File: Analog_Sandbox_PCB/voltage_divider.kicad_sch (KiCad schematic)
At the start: 14 parts, among them J4 PAD, J5 PAD, J6 PAD, J7 PAD

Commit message: Config LM134
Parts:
- S4: footprint Analog_Sandbox_PCB:DS-01 -> Button_Switch_THT:SW_DIP_SPSTx01_Slide_9.78x4.72mm_W7.62mm_P2.54mm

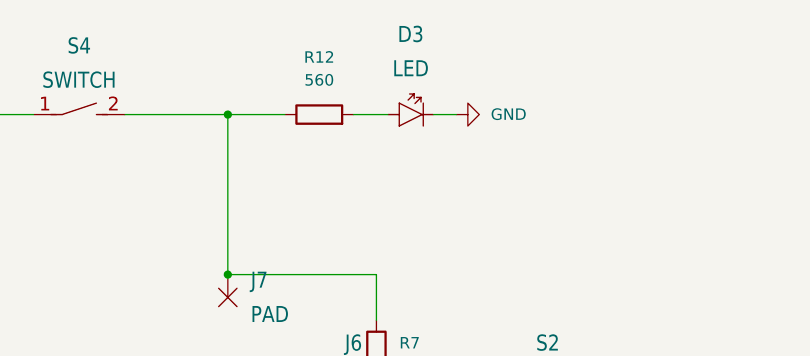
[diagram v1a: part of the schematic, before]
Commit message: All Circuits Added, Layout Almost done
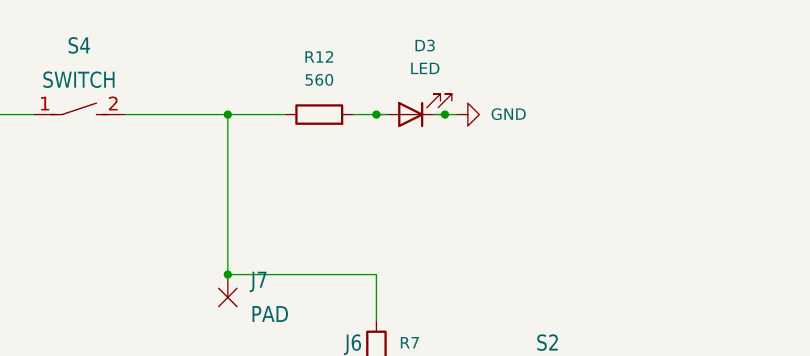
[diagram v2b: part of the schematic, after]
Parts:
- removed D3: LED, Diode_SMD:D_2010_5025Metric_Pad1.52x2.65mm_HandSolder, symbol Analog_Sandbox_PCB-eagle-import:CHIP-FLAT-Y_0603-0.35MM
- added D3: LED, Diode_SMD:D_1206_3216Metric, symbol Device:LED
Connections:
- net GND: now also D3.1 (K)
- net at R12.2: now also D3.2 (A)
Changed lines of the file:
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@@
+	)
+	(junction
+		(at 96.52 26.67)
+		(diameter 0)
+		(color 0 0 0 0)
 	)
 	(junction
@@
 	)
 	(junction
+		(at 104.14 26.67)
+		(diameter 0)
+		(color 0 0 0 0)
+	)
+	(junction
 		(at 80.01 26.67)
 		(diameter 0)
@@
 	(wire
 		(pts
-			(xy 105.41 26.67) (xy 102.87 26.67)
+			(xy 105.41 26.67) (xy 104.14 26.67)
 		)
 		(stroke
@@
 	(wire
 		(pts
+			(xy 96.52 26.67) (xy 97.79 26.67)
+		)
+		(stroke
+			(width 0)
+			(type default)
+		)
+	)
+	(wire
+		(pts
 			(xy 82.55 93.98) (xy 96.52 93.98)
 		)
@@
 	(wire
 		(pts
-			(xy 93.98 26.67) (xy 97.79 26.67)
+			(xy 93.98 26.67) (xy 96.52 26.67)
 		)
 		(stroke
@@
 		(pts
 			(xy 96.52 49.53) (xy 96.52 44.45)
+		)
+		(stroke
+			(width 0)
+			(type default)
+		)
+	)
+	(wire
+		(pts
+			(xy 104.14 26.67) (xy 102.87 26.67)
 		)
 		(stroke
@@
 			)
 			(justify right)
-		)
-	)
-	(symbol
-		(lib_id "Analog_Sandbox_PCB-eagle-import:CHIP-FLAT-Y_0603-0.35MM")
-		(at 100.33 26.67 0)
-		(unit 1)
-		(exclude_from_sim no)
-		(in_bom yes)
-		(on_board yes)
-		(dnp no)
-		(fields_autoplaced yes)
-		(property "Reference" "D3"
-			(at 100.33 17.78 0)
-			(effects
-				(font
-					(size 1.778 1.5113)
-				)
-			)
-		)
-		(property "Value" "LED"
-			(at 100.33 21.59 0)
-			(effects
-				(font
-					(size 1.778 1.5113)
-				)
-			)
-		)
-		(property "Footprint" "Diode_SMD:D_2010_5025Metric_Pad1.52x2.65mm_HandSolder"
-			(at 100.33 26.67 0)
-			(effects
-				(font
-					(size 1.27 1.27)
-				)
-				(hide yes)
-			)
-		)
-		(property "Datasheet" ""
-			(at 100.33 26.67 0)
-			(effects
-				(font
-					(size 1.27 1.27)
-				)
-				(hide yes)
-			)
-		)
-		(property "Description" "Yellow LED - Generic"
-			(at 100.33 26.67 0)
-			(effects
-				(font
-					(size 1.27 1.27)
-				)
-				(hide yes)
-			)
-		)
-		(pin "A"
-		)
-		(pin "C"
-		)
-		(instances
-			(project "Analog_Sandbox_PCB"
-				(path "/ac750111-a1db-4b3c-a106-e1424e47aebb/9c122918-2265-473b-8c84-35fbd0d69d38"
-					(reference "D3")
-					(unit 1)
-				)
-			)
 		)
 	)
@@
 					(unit 1)
 				)
+			)
+		)
+	)
+	(symbol
+		(lib_id "Device:LED")
+		(at 100.33 26.67 180)
+		(unit 1)
+		(exclude_from_sim no)
+		(in_bom yes)
+		(on_board yes)
+		(dnp no)
+		(fields_autoplaced yes)
+		(property "Reference" "D3"
+			(at 101.9175 19.05 0)
+			(effects
+				(font
+					(size 1.27 1.27)
+				)
+			)
+		)
+		(property "Value" "LED"
+			(at 101.9175 21.59 0)
+			(effects
+				(font
+					(size 1.27 1.27)
+				)
+			)
+		)
+		(property "Footprint" "Diode_SMD:D_1206_3216Metric"
+			(at 100.33 26.67 0)
+			(effects
+				(font
+					(size 1.27 1.27)
+				)
+				(hide yes)
+			)
+		)
+		(property "Datasheet" "~"
+			(at 100.33 26.67 0)
+			(effects
+				(font
+					(size 1.27 1.27)
+				)
+				(hide yes)
+			)
+		)
+		(property "Description" "Light emitting diode"
+			(at 100.33 26.67 0)
+			(effects
+				(font
+					(size 1.27 1.27)
+				)
+				(hide yes)
+			)
+		)
+		(property "Sim.Pins" "1=K 2=A"
+			(at 100.33 26.67 0)
+			(effects
+				(font
+					(size 1.27 1.27)
+				)
+				(hide yes)
+			)
+		)
+		(pin "1"
+		)
+		(pin "2"
+		)
+		(instances
+			(project "Analog_Sandbox_PCB"
+				(path "/ac750111-a1db-4b3c-a106-e1424e47aebb/9c122918-2265-473b-8c84-35fbd0d69d38"
+					(reference "D3")
+					(unit 1)
+				)
